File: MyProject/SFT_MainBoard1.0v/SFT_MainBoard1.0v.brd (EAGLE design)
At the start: 100 x 80 mm, 42 parts, among them CN1A ZH, CN1B PH, CN1C XH, CN2A ZH, CN2B PH, CN2C XH, J1 2DC-0005X, M1 SBDBT, X1 ZH04, X2 ZH04, X3 ZH04, X9 ZH

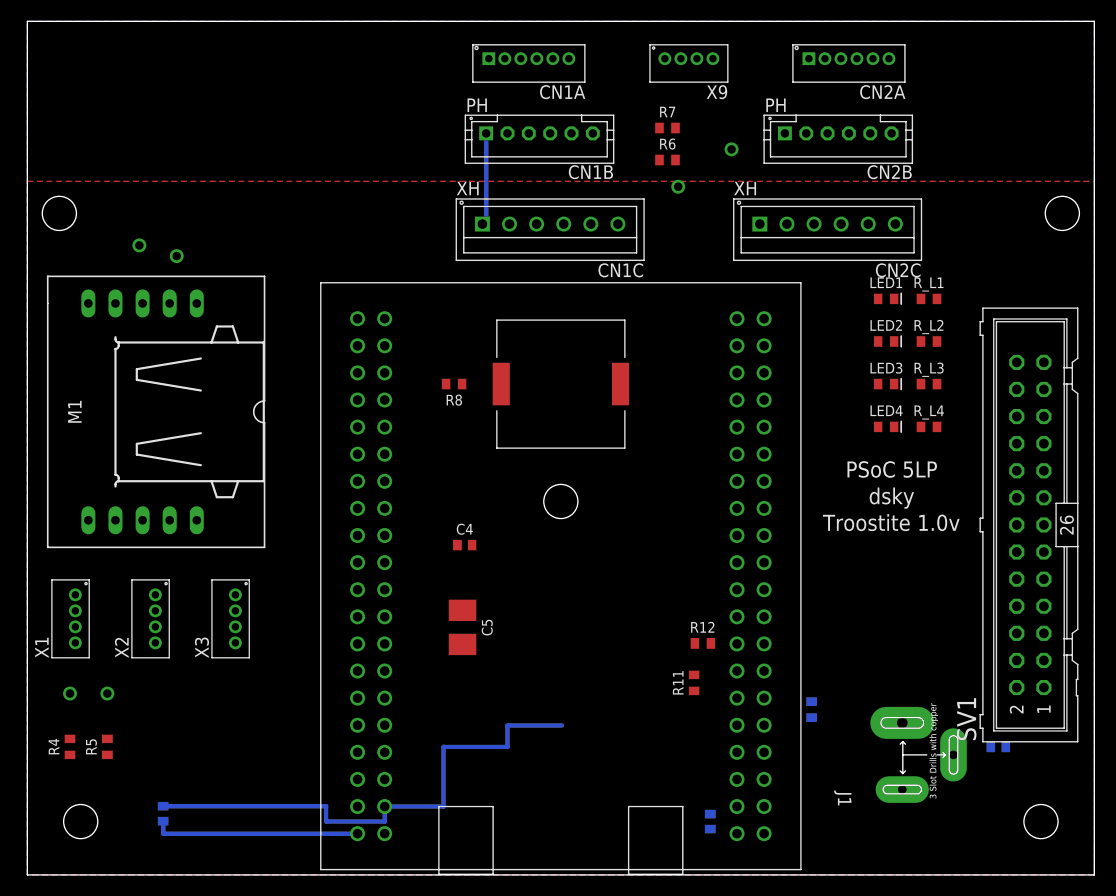
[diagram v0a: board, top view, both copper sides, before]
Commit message: TETUYA KOUSIN
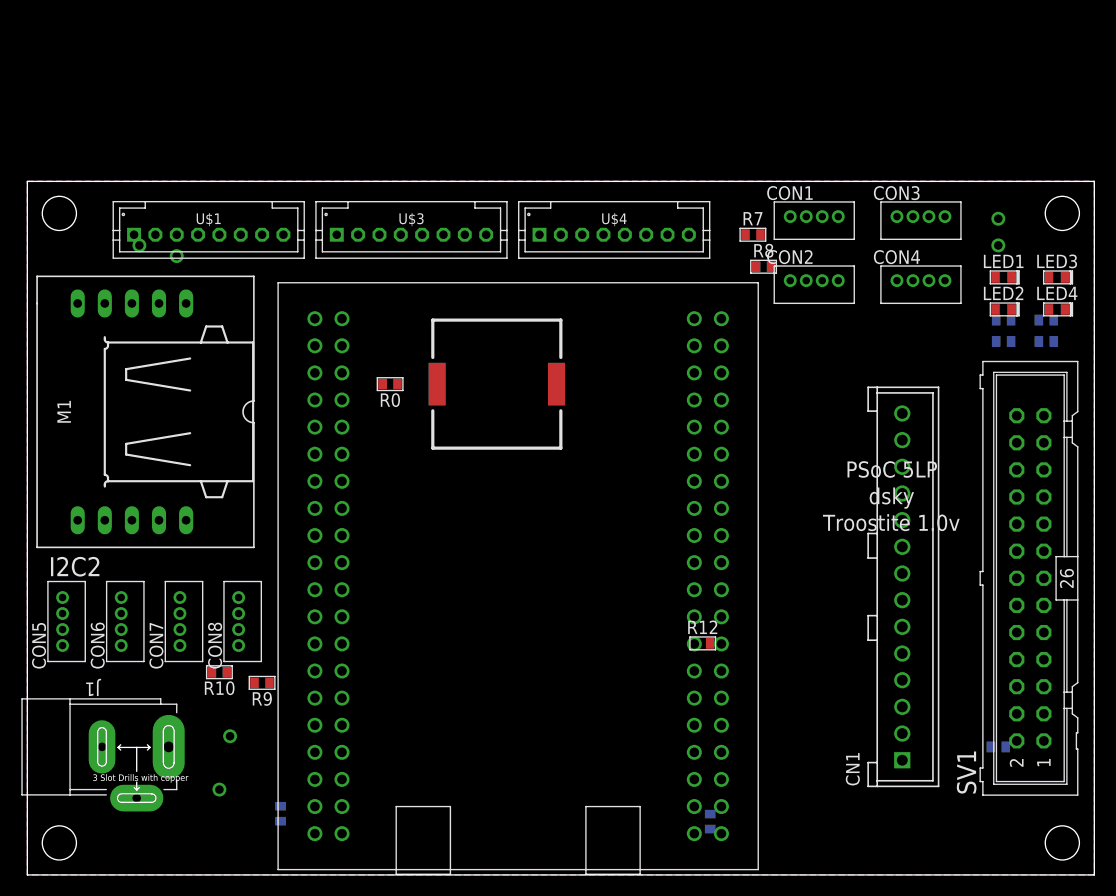
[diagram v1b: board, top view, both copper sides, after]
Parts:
- removed C4: (no value), 02_C:1608
- removed C5: (no value), 02_C:3225
- removed CN1A, CN2A: ZH, jst:B6B-ZR
- removed CN1B, CN2B: PH, jst-ph:JST-PH6
- removed CN1C, CN2C: XH, con-jst-xh:B6B-XH
- removed R11, R5, R6, R_L1, R_L2, R_L3, R_L4: (no value), 01_R:1608
- removed U$76, U$77: CHECK_0.8MM, 08_CONECTOR:CHECK_0.8MM
- removed X1, X2, X3: ZH04, con-jst:B4B-ZR
- removed X9: ZH, con-jst:B4B-ZR
- added CN1: (no value), jst-xa:B14B-XASK-1
- added CON1, CON2, CON3, CON4: I2C1, jst:B4B-ZR
- added CON5, CON6, CON7, CON8: I2C2, jst:B4B-ZR
- added R0, R1, R2, R3, R9: (no value), 01_R:1608
- added U$1, U$3, U$4: JST-PA8, jst-ph:JST-PA8
- added U$15, U$18: CHECK_0.8MM, 08_CONECTOR:CHECK_0.8MM
- moved R4 99.9 mm to (95.5, 52.0), flipped to the bottom, turned to 180 degrees
- moved J1 75.1 mm to (7.00, 12.0), turned to 0 degrees
- moved R10 55.6 mm to (18.0, 19.0), flipped to the top, turned to 0 degrees
- moved R8 31.0 mm to (69.0, 57.0), turned to 180 degrees
- moved U$78 30.1 mm to (91.0, 61.5)
- moved U$79 26.6 mm to (91.0, 59.0)
- moved LED4 19.4 mm to (96.5, 53.0)
- moved LED3 18.9 mm to (96.5, 56.0)
- moved R7 12.8 mm to (68.0, 60.0)
- moved LED2 11.4 mm to (91.5, 53.0)
- moved LED1 11.2 mm to (91.5, 56.0)
- moved C1 11.0 mm to (23.7, 5.74)
- moved U$41 6.00 mm to (44.0, 46.0)
- moved SV1 5.00 mm to (94.0, 27.8)
- moved U$2 4.00 mm to (46.0, 28.0)
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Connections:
- removed net CN1BUS3: CN1A.3, CN1B.3, CN1C.P$3, U$2.P$69
- removed net CN1BUS4: CN1A.4, CN1B.4, CN1C.P$4, U$2.P$67
- removed net CN1BUS5: CN1A.5, CN1B.5, CN1C.P$5, U$2.P$63
- removed net CN1BUS6: CN1A.6, CN1B.6, CN1C.P$6, U$2.P$61
- new net +5V: CON1.2, CON2.2, CON3.2, CON4.2, CON5.2, CON6.2, CON7.2, CON8.2, R10.2, R7.2, R8.2, R9.2
- new net N$10: CON5.3, CON6.3, CON7.3, CON8.3, R9.1, U$18.P$1
- new net N$11: CON5.4, CON6.4, CON7.4, CON8.4, R10.1, U$15.P$1
- new net N$6: CON1.1, CON2.1, CON3.1, CON4.1
- new net N$7: CON5.1, CON6.1, CON7.1, CON8.1
- new net N$8: CON1.3, CON2.3, CON3.3, CON4.3, R8.1, U$79.P$1
- new net N$9: CON1.4, CON2.4, CON3.4, CON4.4, R7.1, U$78.P$1
- net +3.3V: no longer CN1A.2, CN1B.2, CN1C.P$2, CN2A.2, CN2B.2, CN2C.P$2, R4.2, R5.2, R6.2, R7.2, X1.2, X2.2, X3.2, X9.2
- net CN2BUS3: no longer CN2A.3, CN2B.3, CN2C.P$3
- net CN2BUS4: no longer CN2A.4, CN2B.4, CN2C.P$4
- net CN2BUS5: no longer CN2A.5, CN2B.5, CN2C.P$5
- net CN2BUS6: no longer CN2A.6, CN2B.6, CN2C.P$6
- net GND: now also R0.1, R1.1, R2.1, R3.1, R4.1; no longer C4.P$2, C5.P$2, CN1A.1, CN1B.1, CN1C.P$1, CN2A.1, CN2B.1, CN2C.P$1, R8.1, R_L1.1, R_L2.1, R_L3.1, R_L4.1, X1.1, X2.1, X3.1, X9.1
- net N$1: now also R0.2; no longer R8.2
- net N$2: now also R1.2; no longer R_L1.2
- net N$3: now also R2.2; no longer R_L3.2
- net N$4: now also R3.2; no longer R_L4.2
- net N$5: now also R4.2; no longer R_L2.2
- net P12_6: no longer R5.1, U$77.P$1, X1.4, X2.4, X3.4
- net P1_6: no longer R4.1, U$76.P$1, X1.3, X2.3, X3.3
- net P3_0: no longer R10.2
- net P3_2: no longer R10.1
- net P3_5: no longer R11.2
- net P3_7: no longer R11.1
- net P6_1: no longer R6.1, U$78.P$1, X9.3
- net P6_3: no longer R7.1, U$79.P$1, X9.4
- net V_BATT: no longer C4.P$1, C5.P$1
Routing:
- net +3.3V: track 47.8 -> 0.00 mm
- net GND: track 28.2 -> 0.00 mm
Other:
- board size 100 x 80 mm -> 100 x 65 mm
- board text added: "I2C2"
